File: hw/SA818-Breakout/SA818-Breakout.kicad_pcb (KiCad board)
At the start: 2 copper layers, 66 x 53 mm, 32 parts, among them J1 Conn_Coaxial, J2 Conn_01x02, J3 Conn_01x10, Q1 BSS138, Q2 BSS138, Q3 BSS138, Q4 BSS138, U10 NCP1117-5.0_SOT223, U11 NCP1117-3.3_SOT223

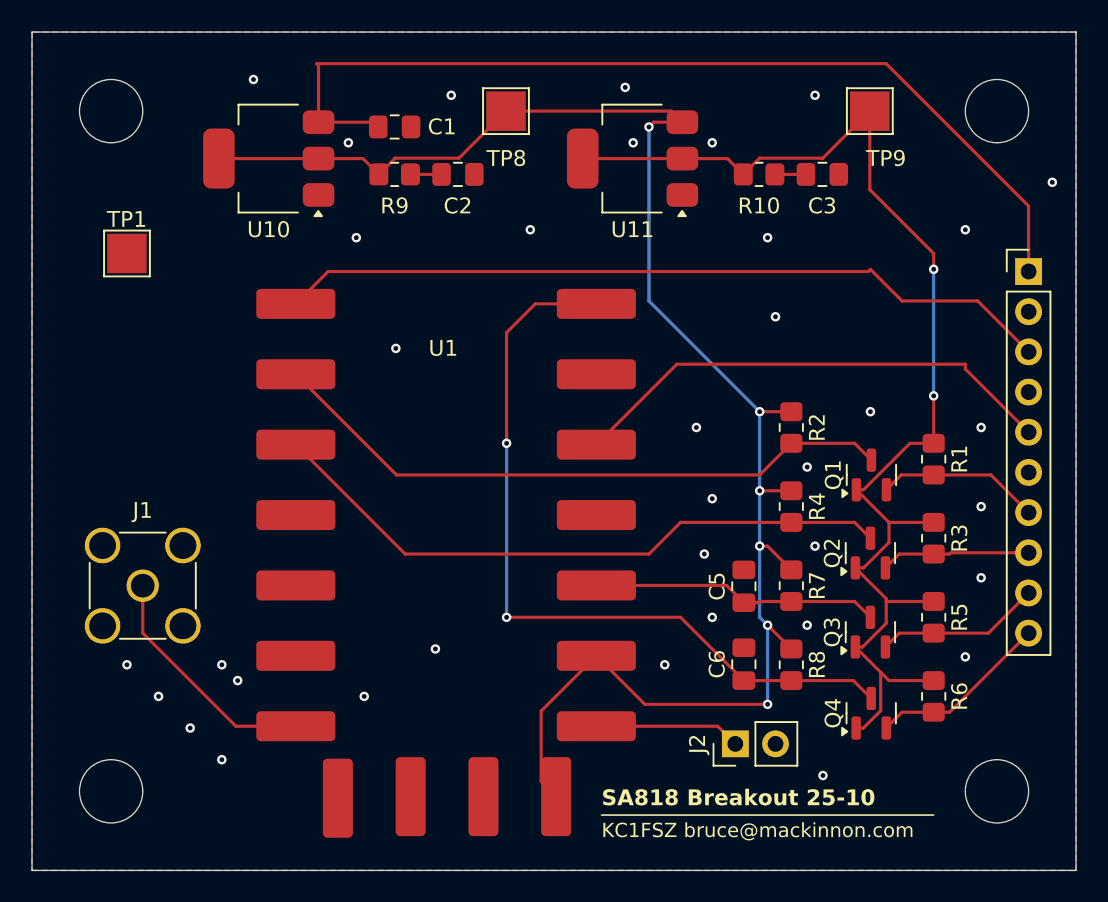
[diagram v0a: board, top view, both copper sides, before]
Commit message: Updating PCB
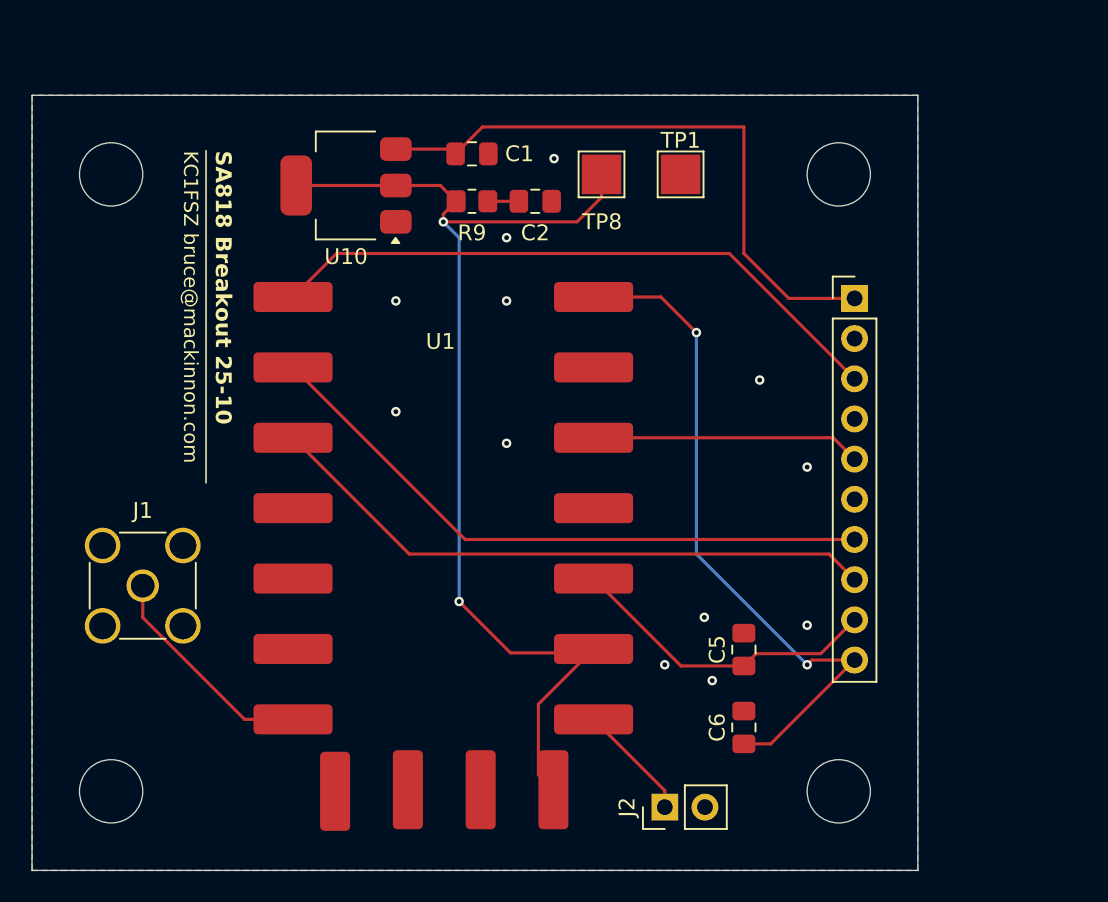
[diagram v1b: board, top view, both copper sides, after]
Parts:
- removed C3: 22u, Capacitor_SMD:C_0805_2012Metric_Pad1.18x1.45mm_HandSolder
- removed Q1, Q2, Q3, Q4: BSS138, Package_TO_SOT_SMD:SOT-23
- removed R1, R2, R3, R4, R5, R6, R7, R8: 10k, Resistor_SMD:R_0805_2012Metric_Pad1.20x1.40mm_HandSolder
- removed R10: 4.7, Resistor_SMD:R_0805_2012Metric_Pad1.20x1.40mm_HandSolder
- removed TP9: TestPoint, TestPoint:TestPoint_Pad_2.5x2.5mm
- removed U11: NCP1117-3.3_SOT223, Package_TO_SOT_SMD:SOT-223-3_TabPin2
- moved TP1 35.4 mm to (144.0, 91.0)
- moved J3 11.1 mm to (155.0, 98.8)
- moved H2 10.8 mm to (154.0, 91.0)
- moved H4 10.0 mm to (154.0, 130.0)
- moved TP8 7.24 mm to (139.0, 91.0)
- moved J2 5.99 mm to (143.0, 131.0)
- moved C1 5.17 mm to (130.8, 89.7)
- moved R9 5.17 mm to (130.8, 92.7)
- moved C2 5.17 mm to (134.8, 92.7)
- moved U10 5.17 mm to (122.8, 91.7)
- moved C5 4.00 mm to (148.0, 121.0)
- moved C6 4.00 mm to (148.0, 126.0)
- moved H1 4.00 mm to (108.0, 91.0)
- moved U1 0.47 mm to (138.5, 98.8)
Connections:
- C5 pad 1: PTT_5 -> PTT_3
- C6 pad 1: AFSQ_5 -> AFSQ_3
- U1 pad 1: AFSQ_5 -> AFSQ_3
- U1 pad 16: RXD_5 -> RXD_3
- U1 pad 17: TXD_5 -> TXD_3
- U1 pad 5: PTT_5 -> PTT_3
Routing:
- net +3.3V: track 78.9 -> 0.00 mm, vias 2 -> 0
- net AFSQ_5: track 49.6 -> 0.00 mm, vias 2 -> 0
- net RXD_5: track 40.4 -> 0.00 mm
- net TXD_5: track 40.3 -> 0.00 mm
- net +5V: track 106.1 -> 69.4 mm, vias 6 -> 2
- net AFSQ_3: track 11.5 -> 43.7 mm, vias 0 -> 2
- net RXD_3: track 9.45 -> 39.2 mm
- net TXD_3: track 10.4 -> 40.0 mm
- net +12V: track 60.5 -> 39.0 mm
- net PTT_5: track 18.2 -> 0.00 mm
- net AF_OUT: track 31.4 -> 17.1 mm
- net PTT_3: track 10.5 -> 20.0 mm
- net AF_IN: track 49.4 -> 39.9 mm
- net Net-(C3-Pad1): track 1.96 -> 0.00 mm
- net Net-(J2-Pin_1): track 9.25 -> 7.41 mm
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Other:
- board size 66 x 53 mm -> 56 x 49 mm
